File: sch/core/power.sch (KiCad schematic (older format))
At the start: 57 parts, among them J1 USB_B_Micro, J2 Reset, J3 V_3.3, J4 CHRG_OUT, J5 V_USB, U1 STM32F427VITx, U2 LM3671-3.3, U3 BQ24296, U4 USBLC6-4SC6, U5 KXO-V97, U6 KXO-V97

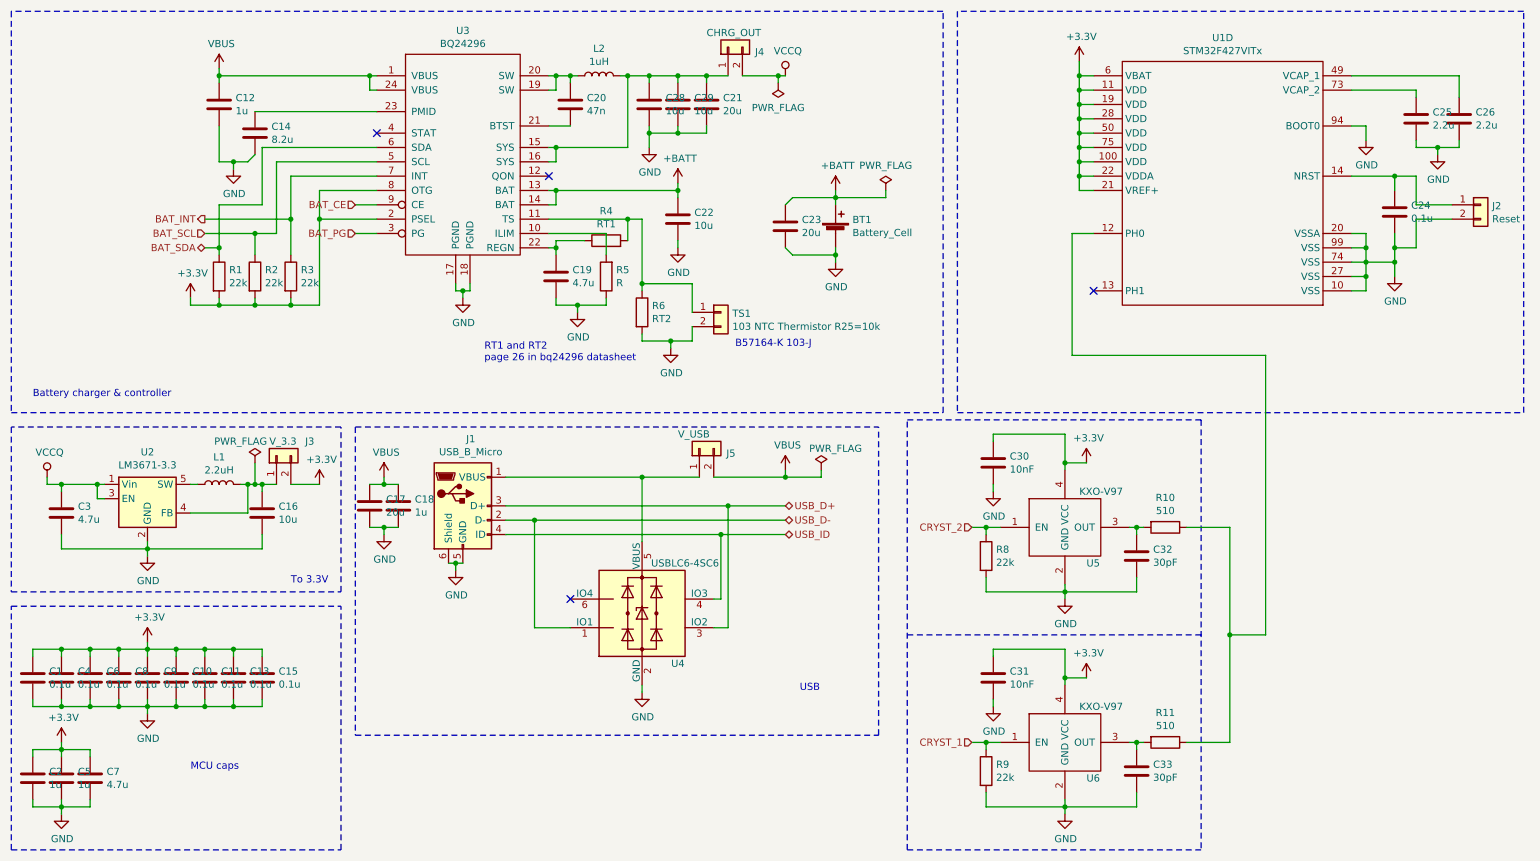
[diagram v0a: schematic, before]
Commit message: new charger schematic
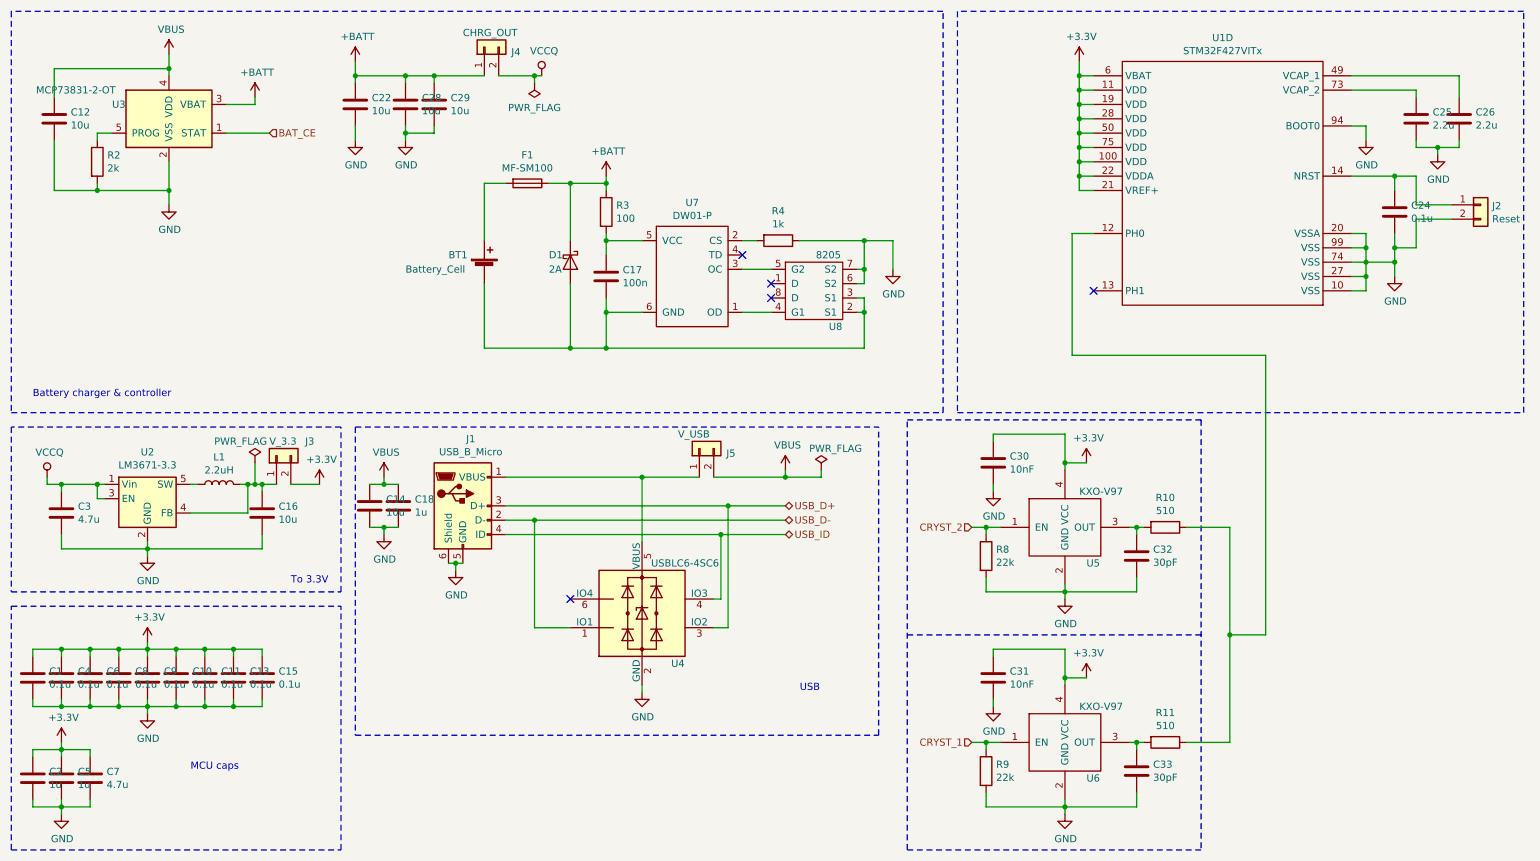
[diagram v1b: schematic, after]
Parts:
- removed C19: 4.7u, Capacitors_SMD:C_0805, symbol Device:C
- removed C20: 47n, Capacitors_SMD:C_0805, symbol Device:C
- removed C21, C23: 20u, Capacitors_SMD:C_1206, symbol Device:C
- removed L2: 1uH, Inductors:Inductor_Taiyo-Yuden_NR-40xx_HandSoldering, symbol Device:L
- removed R1: 22k, Resistors_SMD:R_0603, symbol Device:R
- removed R5: R, Resistors_SMD:R_0603, symbol Device:R
- removed R6: RT2, Resistors_SMD:R_0603, symbol Device:R
- removed TS1: 103 NTC Thermistor R25=10k, Connector_PinHeader_1.27mm:PinHeader_1x02_P1.27mm_Vertical, symbol Connector_Generic:Conn_01x02
- removed U3: BQ24296, Housings_DFN_QFN:QFN-24_4x4mm_Pitch0.5mm, symbol core-rescue:BQ24296-core
- added D1: 2A, Diode_SMD:D_2010_5025Metric, symbol Device:D_Schottky
- added F1: MF-SM100, Fuse:Fuse_Bourns_MF-SM_9.5x6.71mm, symbol Device:Fuse
- added U3: MCP73831-2-OT, Package_TO_SOT_SMD:SOT-23-5, symbol Battery_Management:MCP73831-2-OT
- added U7: DW01-P, Package_TO_SOT_SMD:SOT-23-6, symbol core-rescue:DW01-P
- added U8: 8205, Package_SO:TSSOP-8_4.4x3mm_P0.65mm, symbol core-rescue:8205
- C12: value 1u -> 10u
- C14: value 8.2u -> 10u
- C17: value 20u -> 100n; footprint Capacitors_SMD:C_1206 -> Capacitor_SMD:C_0402_1005Metric
- R2: value 22k -> 2k; footprint Resistors_SMD:R_0603 -> Resistor_SMD:R_0603_1608Metric_Pad1.05x0.95mm_HandSolder
- R3: value 22k -> 100; footprint Resistors_SMD:R_0603 -> Resistor_SMD:R_0603_1608Metric_Pad1.05x0.95mm_HandSolder
- R4: value RT1 -> 1k; footprint Resistors_SMD:R_0603 -> Resistor_SMD:R_0603_1608Metric_Pad1.05x0.95mm_HandSolder
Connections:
- net BAT_INT is gone; now on net +BATT: R3.1
- net +3V3: no longer R2.2, R3.2
- net +BATT: now also C28.1, C29.1, J4.1 (Pin_1), D1.1 (K), F1.1, U3.3 (VBAT); no longer BT1.1 (+)
- net BAT_CE: now also U3.1 (STAT)
- net GND: now also R2.2, R4.1, U3.2 (VSS), U8.6 (S2), U8.7 (S2); no longer BT1.2 (-), C17.2
- net VBUS: now also C14.1, U3.4 (VDD); no longer C17.1
- net at R4.2: now also U7.2 (CS)
- net BAT_SCL: no longer names the net of R2.1
- net BAT_SCL: now also U3.5 (PROG)
- new net: BT1.1 (+), F1.2
- new net: BT1.2 (-), C17.2, D1.2 (A), U7.6 (GND), U8.2 (S1), U8.3 (S1)
- new net: U7.1 (OD), U8.4 (G1)
- new net: U7.3 (OC), U8.5 (G2)
- new net: C17.1, R3.2, U7.5 (VCC)
- no-connect marks 4 -> 5
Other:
- note removed: "B57164-K 103-J"
- note removed: "RT1 and RT2\npage 26 in bq24296 datasheet"
- moved on the sheet: BT1, C22, C28, C29, J4
